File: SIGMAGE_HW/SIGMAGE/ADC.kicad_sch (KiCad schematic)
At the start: 68 parts, among them J10 SJ63073E, J11 SJ63073E, J2 SJ63073E, J4 SJ63073E, U16 OPA1612AIDRGR, U17 OPA1612AIDRGR, U18 PCM1803ADB, U19 PCM1803ADB, U4 OPA1612AIDRGR, U5 PCM1803ADB, U6 OPA1612AIDRGR, U7 PCM1803ADB

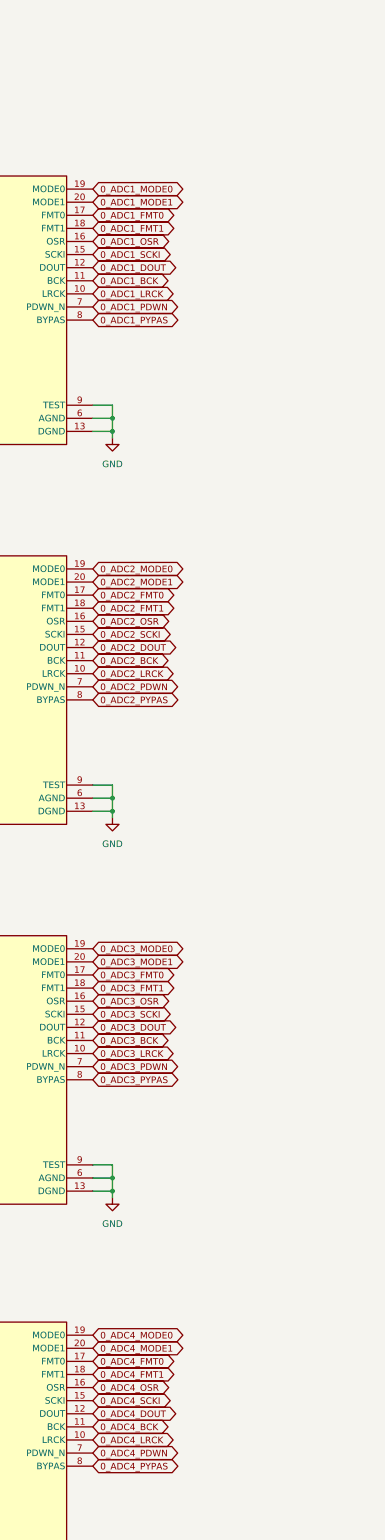
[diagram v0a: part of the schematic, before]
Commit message: improvements
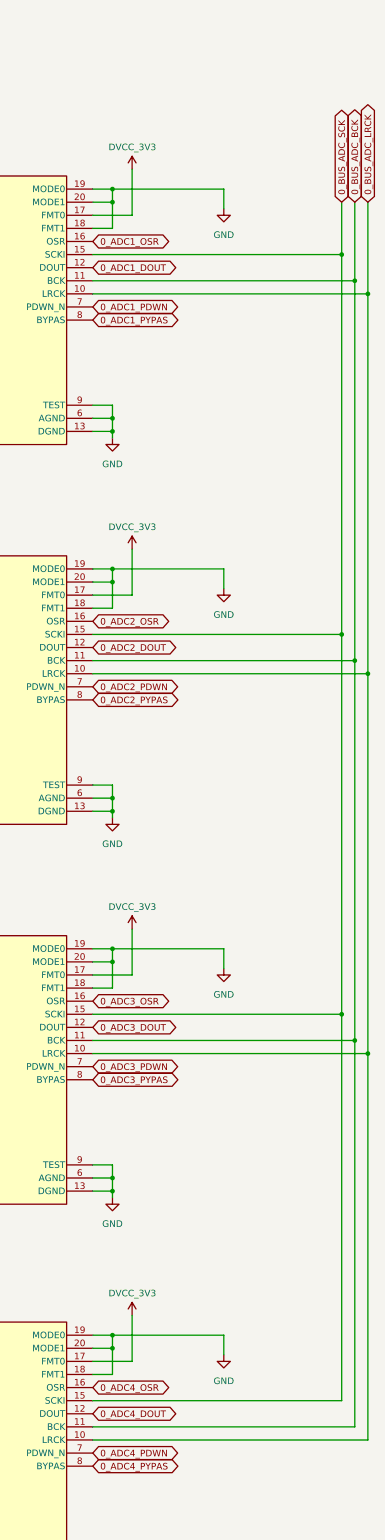
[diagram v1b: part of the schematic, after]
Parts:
- C12, C125, C126, C127, C128, C129, C13, C130, C131, C132, C133, C134, C135, C136, C137, C138, C139, C140, C141, C142, C173, C174, C175, C176, C179, C18, C180, C181, C182, C183, C184, C185, C186, C19, C20, C21, C22, C23, C89, C90: footprint Resistor_SMD:R_0603_1608Metric -> Capacitor_SMD:C_0603_1608Metric
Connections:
- net 0_ADC1_FMT0 is gone; now on net DVCC_3V3: U5.17 (FMT0)
- net 0_ADC1_FMT1 is gone; now on net GND: U5.18 (FMT1)
- net 0_ADC1_MODE0 is gone; now on net GND: U5.19 (MODE0)
- net 0_ADC1_MODE1 is gone; now on net GND: U5.20 (MODE1)
- net 0_ADC2_BCK is gone; now on net 0_BUS_ADC_BCK: U7.11 (BCK)
- net 0_ADC2_FMT0 is gone; now on net DVCC_3V3: U7.17 (FMT0)
- net 0_ADC2_FMT1 is gone; now on net GND: U7.18 (FMT1)
- net 0_ADC2_LRCK is gone; now on net 0_BUS_ADC_LRCK: U7.10 (LRCK)
- net 0_ADC2_MODE0 is gone; now on net GND: U7.19 (MODE0)
- net 0_ADC2_MODE1 is gone; now on net GND: U7.20 (MODE1)
- net 0_ADC2_SCKI is gone; now on net 0_BUS_ADC_SCK: U7.15 (SCKI)
- net 0_ADC3_BCK is gone; now on net 0_BUS_ADC_BCK: U18.11 (BCK)
- net 0_ADC3_FMT0 is gone; now on net DVCC_3V3: U18.17 (FMT0)
- net 0_ADC3_FMT1 is gone; now on net GND: U18.18 (FMT1)
- net 0_ADC3_LRCK is gone; now on net 0_BUS_ADC_LRCK: U18.10 (LRCK)
- net 0_ADC3_MODE0 is gone; now on net GND: U18.19 (MODE0)
- net 0_ADC3_MODE1 is gone; now on net GND: U18.20 (MODE1)
- net 0_ADC3_SCKI is gone; now on net 0_BUS_ADC_SCK: U18.15 (SCKI)
- net 0_ADC4_BCK is gone; now on net 0_BUS_ADC_BCK: U19.11 (BCK)
- net 0_ADC4_FMT0 is gone; now on net DVCC_3V3: U19.17 (FMT0)
- net 0_ADC4_FMT1 is gone; now on net GND: U19.18 (FMT1)
- net 0_ADC4_LRCK is gone; now on net 0_BUS_ADC_LRCK: U19.10 (LRCK)
- net 0_ADC4_MODE0 is gone; now on net GND: U19.19 (MODE0)
- net 0_ADC4_MODE1 is gone; now on net GND: U19.20 (MODE1)
- net 0_ADC4_SCKI is gone; now on net 0_BUS_ADC_SCK: U19.15 (SCKI)
- net 0_ADC1_BCK renamed 0_BUS_ADC_BCK
- net 0_ADC1_LRCK renamed 0_BUS_ADC_LRCK
- net 0_ADC1_SCKI renamed 0_BUS_ADC_SCK
